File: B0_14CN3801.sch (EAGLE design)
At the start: 19 parts

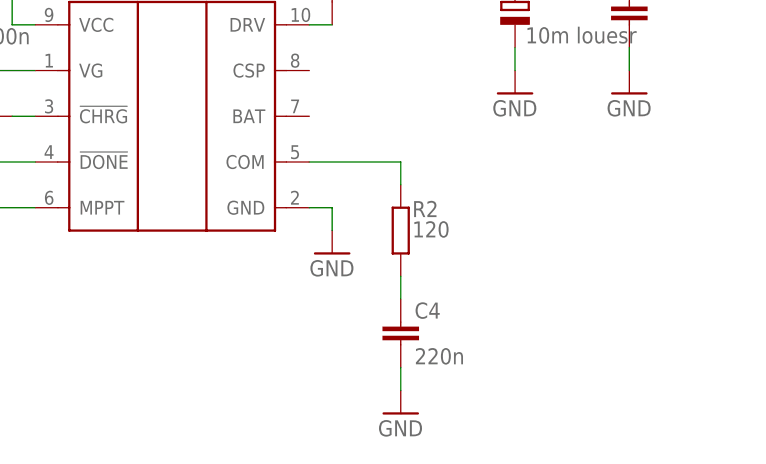
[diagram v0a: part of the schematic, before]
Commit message: .
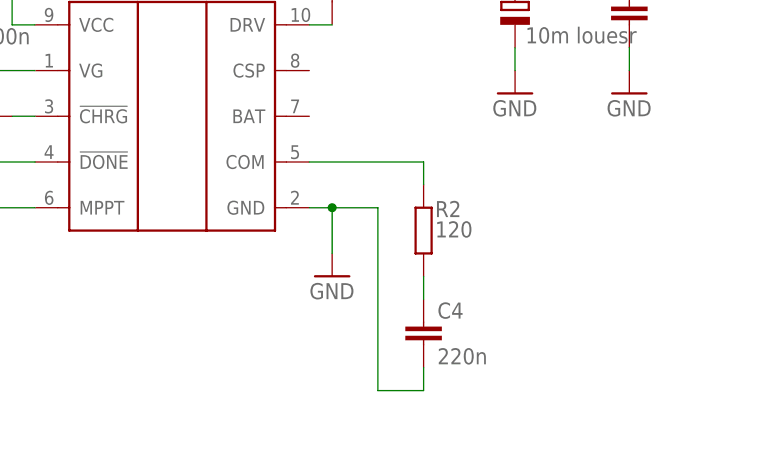
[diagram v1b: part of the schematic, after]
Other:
- moved on the sheet: C4, R2
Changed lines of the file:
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@@
 <part name="C1" library="rcl" deviceset="C-EU" device="C0805" value="100n"/>
 <part name="GND1" library="supply1v" deviceset="GND" device=""/>
-<part name="GND2" library="supply1v" deviceset="GND" device=""/>
 <part name="HL1" library="led" deviceset="LED" device="CHIPLED_0603"/>
 <part name="HL2" library="led" deviceset="LED" device="CHIPLED_0603"/>
@@
 </instance>
 <instance part="GND1" gate="1" x="-12.7" y="53.34"/>
-<instance part="GND2" gate="1" x="50.8" y="35.56"/>
 <instance part="HL1" gate="G$1" x="10.16" y="50.8" smashed="yes" rot="R90">
 <attribute name="NAME" x="12.192" y="54.356" size="1.778" layer="95" rot="R180"/>
@@
 <attribute name="VALUE" x="5.842" y="57.15" size="1.778" layer="96" rot="R90"/>
 </instance>
-<instance part="R2" gate="G$1" x="58.42" y="38.1" smashed="yes" rot="R90">
-<attribute name="NAME" x="59.69" y="39.5986" size="1.778" layer="95"/>
-<attribute name="VALUE" x="59.69" y="37.338" size="1.778" layer="96"/>
+<instance part="R2" gate="G$1" x="60.96" y="38.1" smashed="yes" rot="R90">
+<attribute name="NAME" x="62.23" y="39.5986" size="1.778" layer="95"/>
+<attribute name="VALUE" x="62.23" y="37.338" size="1.778" layer="96"/>
 </instance>
 <instance part="R3" gate="G$1" x="-5.08" y="53.34" smashed="yes" rot="R90">
@@
 </instance>
 <instance part="GND3" gate="1" x="-5.08" y="22.86"/>
-<instance part="C4" gate="G$1" x="58.42" y="27.94"/>
-<instance part="GND4" gate="1" x="58.42" y="17.78"/>
+<instance part="C4" gate="G$1" x="60.96" y="27.94"/>
+<instance part="GND4" gate="1" x="50.8" y="33.02"/>
 <instance part="VT1" gate="G$1" x="53.34" y="66.04" smashed="yes" rot="R90">
 <attribute name="NAME" x="50.8" y="71.12" size="1.778" layer="95"/>
@@
 <net name="GND" class="0">
 <segment>
-<pinref part="DA1" gate="DA" pin="GND"/>
-<wire x1="48.26" y1="40.64" x2="50.8" y2="40.64" width="0.1524" layer="91"/>
-<pinref part="GND2" gate="1" pin="GND"/>
-<wire x1="50.8" y1="40.64" x2="50.8" y2="38.1" width="0.1524" layer="91"/>
-</segment>
-<segment>
 <pinref part="C1" gate="G$1" pin="2"/>
 <pinref part="GND1" gate="1" pin="GND"/>
@@
 <pinref part="C4" gate="G$1" pin="2"/>
 <pinref part="GND4" gate="1" pin="GND"/>
-<wire x1="58.42" y1="22.86" x2="58.42" y2="20.32" width="0.1524" layer="91"/>
+<wire x1="55.88" y1="20.32" x2="55.88" y2="40.64" width="0.1524" layer="91"/>
+<pinref part="DA1" gate="DA" pin="GND"/>
+<wire x1="55.88" y1="40.64" x2="50.8" y2="40.64" width="0.1524" layer="91"/>
+<wire x1="50.8" y1="40.64" x2="48.26" y2="40.64" width="0.1524" layer="91"/>
+<wire x1="50.8" y1="35.56" x2="50.8" y2="40.64" width="0.1524" layer="91"/>
+<wire x1="55.88" y1="20.32" x2="60.96" y2="20.32" width="0.1524" layer="91"/>
+<wire x1="60.96" y1="20.32" x2="60.96" y2="22.86" width="0.1524" layer="91"/>
+<junction x="50.8" y="40.64"/>
 </segment>
 <segment>
@@
 <segment>
 <pinref part="DA1" gate="DA" pin="COM"/>
-<wire x1="48.26" y1="45.72" x2="58.42" y2="45.72" width="0.1524" layer="91"/>
+<wire x1="48.26" y1="45.72" x2="60.96" y2="45.72" width="0.1524" layer="91"/>
 <pinref part="R2" gate="G$1" pin="2"/>
-<wire x1="58.42" y1="45.72" x2="58.42" y2="43.18" width="0.1524" layer="91"/>
+<wire x1="60.96" y1="45.72" x2="60.96" y2="43.18" width="0.1524" layer="91"/>
 </segment>
 </net>
@@
 <segment>
 <pinref part="R2" gate="G$1" pin="1"/>
-<wire x1="58.42" y1="33.02" x2="58.42" y2="30.48" width="0.1524" layer="91"/>
+<wire x1="60.96" y1="33.02" x2="60.96" y2="30.48" width="0.1524" layer="91"/>
 <pinref part="C4" gate="G$1" pin="1"/>
 </segment>
